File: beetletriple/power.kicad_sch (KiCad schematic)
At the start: 20 parts, among them U1 TPS54331DR, U2 HT7550-1

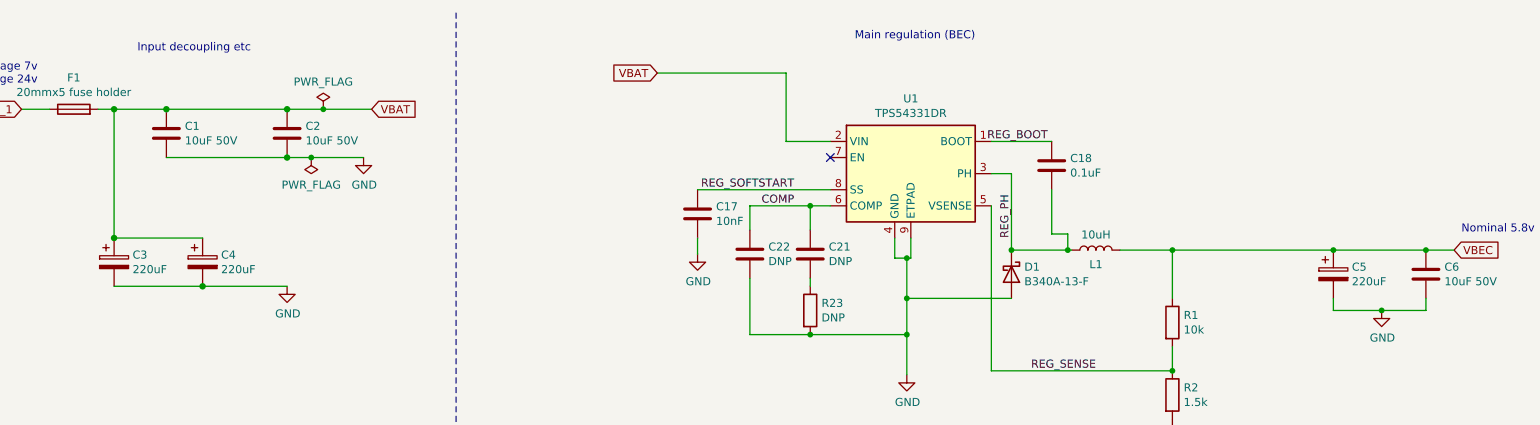
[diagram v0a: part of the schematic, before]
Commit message: misc updates
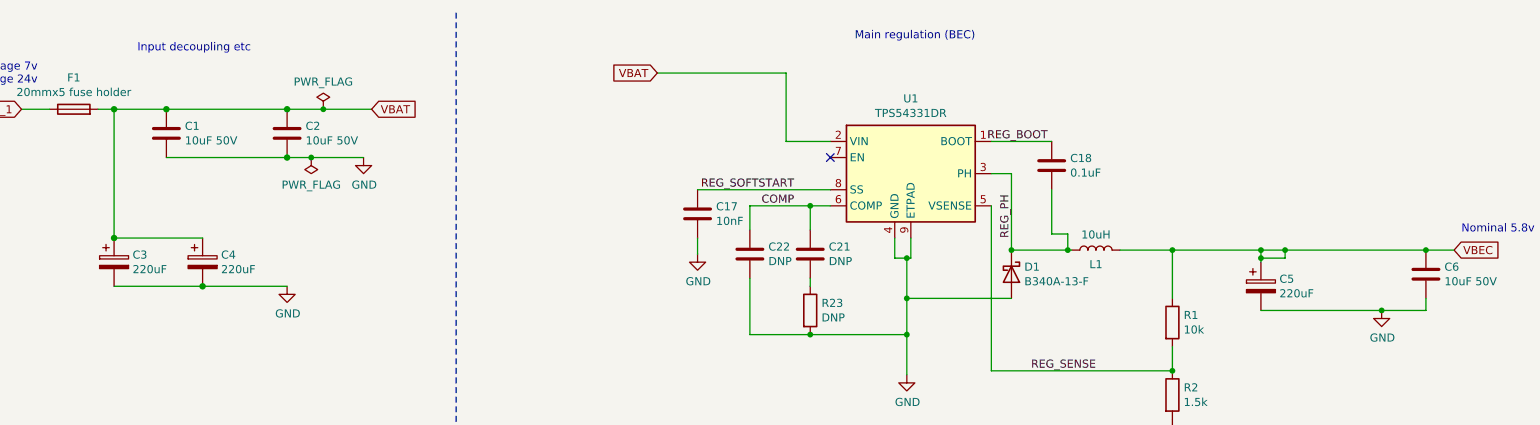
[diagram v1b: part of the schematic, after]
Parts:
- removed C5: 220uF, Capacitor_SMD:C_Elec_10x10.2, symbol Device:C_Polarized
- added C5: 220uF, Capacitor_SMD:C_Elec_10x10.2, symbol Device:CP
- C3, C4: symbol Device:C_Polarized -> Device:CP
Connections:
- net GND: now also C5.2
- net VBEC: now also C5.1
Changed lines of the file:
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@@
   (junction (at 210.185 60.96) (diameter 0.9144) (color 0 0 0 0))
   (junction (at 210.185 80.01) (diameter 0.9144) (color 0 0 0 0))
-  (junction (at 235.585 60.96) (diameter 0.9144) (color 0 0 0 0))
+  (junction (at 224.155 60.96) (diameter 0.9144) (color 0 0 0 0))
+  (junction (at 224.155 62.23) (diameter 0.9144) (color 0 0 0 0))
+  (junction (at 227.965 60.96) (diameter 0.9144) (color 0 0 0 0))
   (junction (at 243.205 70.485) (diameter 0.9144) (color 0 0 0 0))
   (junction (at 250.19 60.96) (diameter 0.9144) (color 0 0 0 0))
@@
     (stroke (width 0) (type solid) (color 0 0 0 0))
   )
-  (wire (pts (xy 43.18 38.735) (xy 51.435 38.735))
-    (stroke (width 0) (type solid) (color 0 0 0 0))
-  )
   (wire (pts (xy 43.18 59.055) (xy 57.15 59.055))
     (stroke (width 0) (type solid) (color 0 0 0 0))
@@
     (stroke (width 0) (type solid) (color 0 0 0 0))
   )
+  (wire (pts (xy 51.435 38.735) (xy 43.18 38.735))
+    (stroke (width 0) (type solid) (color 0 0 0 0))
+  )
   (wire (pts (xy 51.435 38.735) (xy 70.485 38.735))
     (stroke (width 0) (type solid) (color 0 0 0 0))
@@
     (stroke (width 0) (type solid) (color 0 0 0 0))
   )
-  (wire (pts (xy 70.485 46.355) (xy 74.295 46.355))
+  (wire (pts (xy 74.295 46.355) (xy 70.485 46.355))
     (stroke (width 0) (type solid) (color 0 0 0 0))
   )
@@
     (stroke (width 0) (type solid) (color 0 0 0 0))
   )
-  (wire (pts (xy 168.275 62.23) (xy 168.275 68.58))
-    (stroke (width 0) (type solid) (color 0 0 0 0))
-  )
   (wire (pts (xy 168.275 62.23) (xy 168.91 62.23))
     (stroke (width 0) (type solid) (color 0 0 0 0))
   )
+  (wire (pts (xy 168.275 68.58) (xy 168.275 62.23))
+    (stroke (width 0) (type solid) (color 0 0 0 0))
+  )
   (wire (pts (xy 168.275 74.295) (xy 168.275 68.58))
     (stroke (width 0) (type solid) (color 0 0 0 0))
@@
     (stroke (width 0) (type solid) (color 0 0 0 0))
   )
-  (wire (pts (xy 184.785 60.96) (xy 193.675 60.96))
-    (stroke (width 0) (type solid) (color 0 0 0 0))
-  )
   (wire (pts (xy 184.785 68.58) (xy 168.275 68.58))
     (stroke (width 0) (type solid) (color 0 0 0 0))
@@
     (stroke (width 0) (type solid) (color 0 0 0 0))
   )
+  (wire (pts (xy 193.675 60.96) (xy 184.785 60.96))
+    (stroke (width 0) (type solid) (color 0 0 0 0))
+  )
   (wire (pts (xy 193.675 60.96) (xy 194.31 60.96))
     (stroke (width 0) (type solid) (color 0 0 0 0))
@@
     (stroke (width 0) (type solid) (color 0 0 0 0))
   )
-  (wire (pts (xy 210.185 60.96) (xy 235.585 60.96))
+  (wire (pts (xy 210.185 60.96) (xy 250.19 60.96))
     (stroke (width 0) (type solid) (color 0 0 0 0))
   )
@@
     (stroke (width 0) (type solid) (color 0 0 0 0))
   )
-  (wire (pts (xy 235.585 60.96) (xy 250.19 60.96))
-    (stroke (width 0) (type solid) (color 0 0 0 0))
-  )
-  (wire (pts (xy 235.585 68.58) (xy 235.585 70.485))
-    (stroke (width 0) (type solid) (color 0 0 0 0))
-  )
-  (wire (pts (xy 235.585 70.485) (xy 243.205 70.485))
+  (wire (pts (xy 224.155 60.96) (xy 224.155 62.23))
+    (stroke (width 0) (type solid) (color 0 0 0 0))
+  )
+  (wire (pts (xy 224.155 62.23) (xy 224.155 62.865))
+    (stroke (width 0) (type solid) (color 0 0 0 0))
+  )
+  (wire (pts (xy 224.155 62.23) (xy 227.965 62.23))
+    (stroke (width 0) (type solid) (color 0 0 0 0))
+  )
+  (wire (pts (xy 224.155 70.485) (xy 243.205 70.485))
+    (stroke (width 0) (type solid) (color 0 0 0 0))
+  )
+  (wire (pts (xy 227.965 60.96) (xy 227.965 62.23))
     (stroke (width 0) (type solid) (color 0 0 0 0))
   )
@@
   (symbol (lib_id "power:PWR_FLAG") (at 74.295 46.355 180) (unit 1)
     (in_bom yes) (on_board yes)
-    (property "Reference" "#FLG?" (id 0) (at 74.295 48.26 0)
+    (property "Reference" "#FLG01" (id 0) (at 74.295 48.26 0)
       (effects (font (size 1.27 1.27)) hide)
     )
@@
     (pin "2")
   )
-  (symbol (lib_id "Device:C_Polarized") (at 43.18 62.865 0) (unit 1)
+  (symbol (lib_id "Device:CP") (at 43.18 62.865 0) (unit 1)
     (in_bom yes) (on_board yes)
     (property "Reference" "C3" (id 0) (at 46.1011 61.7156 0)
@@
     (pin "2")
   )
-  (symbol (lib_id "Device:C_Polarized") (at 57.15 62.865 0) (unit 1)
+  (symbol (lib_id "Device:CP") (at 57.15 62.865 0) (unit 1)
     (in_bom yes) (on_board yes)
     (property "Reference" "C4" (id 0) (at 60.0711 61.7156 0)
@@
     (pin "2")
   )
-  (symbol (lib_id "Device:C_Polarized") (at 235.585 64.77 0) (unit 1)
-    (in_bom yes) (on_board yes)
-    (property "Reference" "C5" (id 0) (at 238.5061 63.6206 0)
-      (effects (font (size 1.27 1.27)) (justify left))
-    )
-    (property "Value" "220uF" (id 1) (at 238.506 65.919 0)
-      (effects (font (size 1.27 1.27)) (justify left))
-    )
-    (property "Footprint" "Capacitor_SMD:C_Elec_10x10.2" (id 2) (at 236.5502 68.58 0)
-      (effects (font (size 1.27 1.27)) hide)
-    )
-    (property "Datasheet" "~" (id 3) (at 235.585 64.77 0)
-      (effects (font (size 1.27 1.27)) hide)
-    )
-    (property "LCSC" "C125977" (id 4) (at 235.585 64.77 0)
-      (effects (font (size 1.27 1.27)) hide)
-    )
+  (symbol (lib_id "Device:CP") (at 224.155 66.675 0) (unit 1)
+    (in_bom yes) (on_board yes)
+    (property "Reference" "C5" (id 0) (at 227.076 65.526 0)
+      (effects (font (size 1.27 1.27)) (justify left))
+    )
+    (property "Value" "220uF" (id 1) (at 227.076 67.824 0)
+      (effects (font (size 1.27 1.27)) (justify left))
+    )
+    (property "Footprint" "Capacitor_SMD:C_Elec_10x10.2" (id 2) (at 225.1202 70.485 0)
+      (effects (font (size 1.27 1.27)) hide)
+    )
+    (property "Datasheet" "~" (id 3) (at 224.155 66.675 0)
+      (effects (font (size 1.27 1.27)) hide)
+    )
+    (property "LCSC" "C125977" (id 4) (at 224.155 66.675 0)
+      (effects (font (size 1.27 1.27)) hide)
+    )
